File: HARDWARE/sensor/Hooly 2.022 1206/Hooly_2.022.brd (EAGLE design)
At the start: 33.4 x 25.4 mm, 34 parts, among them IC2 MCP1703CB, U3 MCP73831, U5 ATMEGA328P-AU

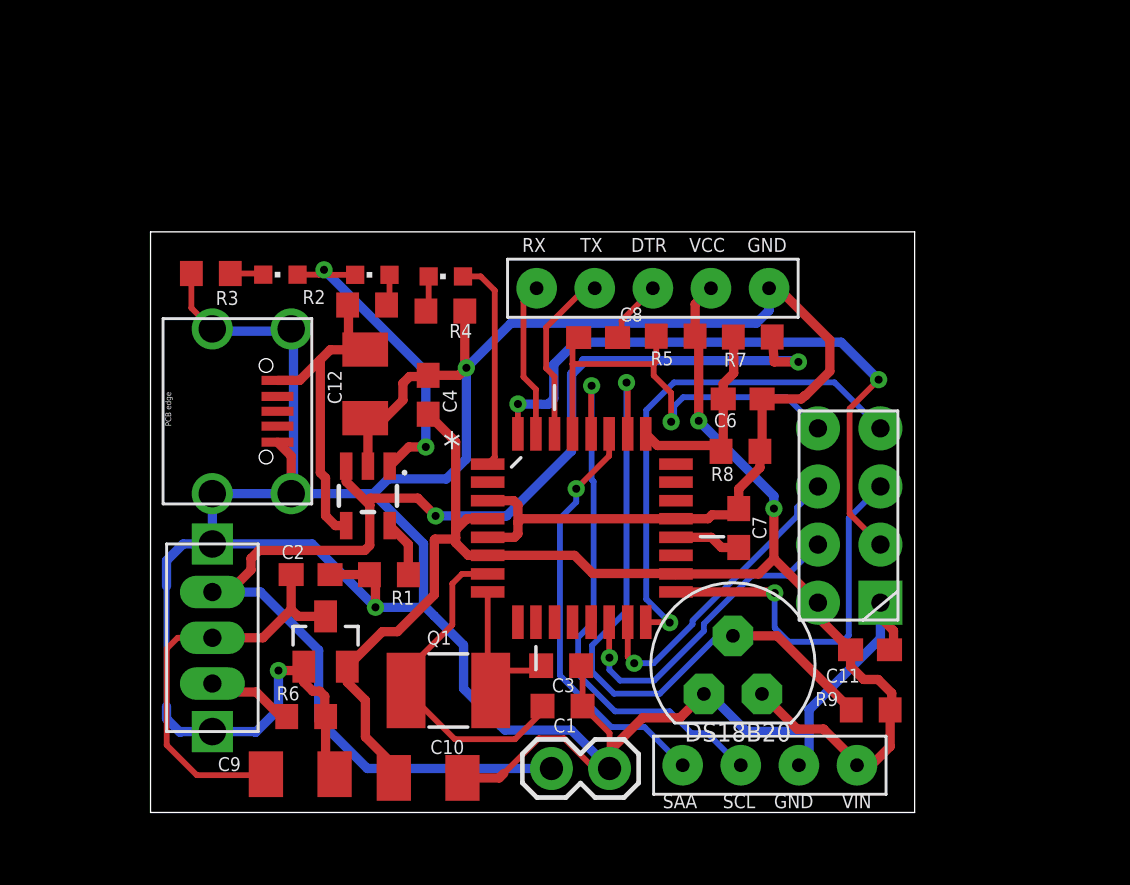
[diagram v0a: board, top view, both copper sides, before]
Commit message: Hardware update
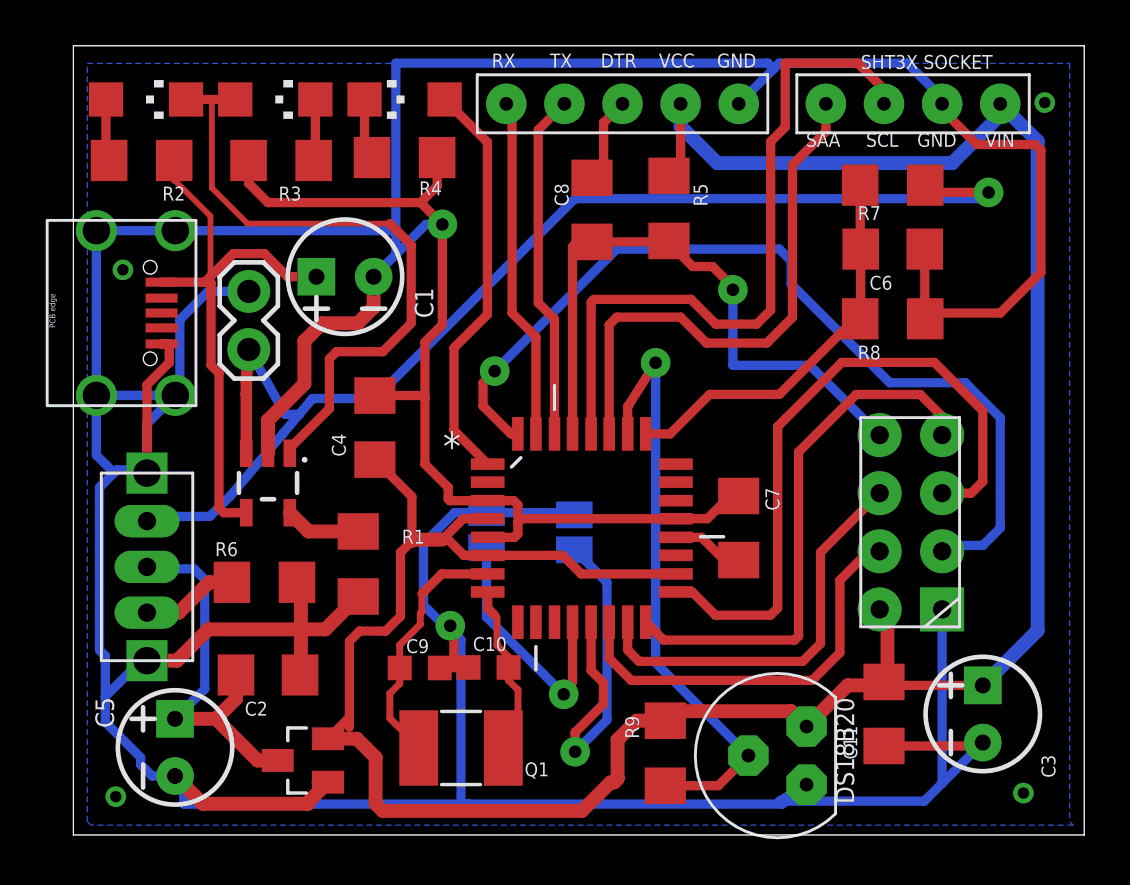
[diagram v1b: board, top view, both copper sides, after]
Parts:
- removed C12: (no value), resistor:C1206K
- added C5: 10uF, SparkFun-Capacitors:CPOL-RADIAL-2.5MM-5MM
- added SJ1, SJ2: (no value), jumper:SJ
- C1: value (none) -> 4.7uF; device rcl:C0603K -> SparkFun-Capacitors:CPOL-RADIAL-2.5MM-5MM
- C10, C9: value 1uF -> 22pF; device resistor:C1206K -> rcl:C0603K
- C11, C2, C4, C6, C7, C8: device resistor:C0603 -> resistor:C1206
- C3: value (none) -> 10uF; device rcl:C0603K -> SparkFun-Capacitors:CPOL-RADIAL-2.5MM-5MM
- LED1, LED2, LED4: device led:CHIPLED_0603 -> led:CHIPLED_1206
- Q1: value (none) -> 8MHz Crystal
- R1, R2, R3, R4, R5, R6, R7, R8, R9: device rcl:R0603 -> rcl:R1206
- moved U$1 29.6 mm to (34.8, 30.0)
- moved J2 26.1 mm to (8.30, 21.8), turned to 270 degrees
- moved C1 21.0 mm to (12.5, 22.4), turned to 180 degrees
- moved C3 18.6 mm to (40.4, 3.30), turned to 90 degrees
- moved LED1 12.5 mm to (3.81, 30.2), turned to 270 degrees
- moved R2 11.7 mm to (3.62, 27.5), turned to 180 degrees
- moved C6 9.27 mm to (36.4, 23.6)
- moved R9 9.18 mm to (26.5, 1.59), turned to 90 degrees
- moved R7 9.03 mm to (36.4, 26.4)
- moved R8 8.82 mm to (36.4, 20.6)
- moved U$6 8.17 mm to (20.8, 30.0)
- moved LED4 7.94 mm to (15.1, 30.2)
- moved LED2 7.66 mm to (9.46, 30.2), turned to 270 degrees
- moved C9 6.99 mm to (15.8, 5.31)
- moved R4 6.94 mm to (15.1, 27.6)
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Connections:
- net GND: now also C10.1, C3.2, C5.2, SJ1.1, SJ2.2; no longer C10.2, C12.2, C3.1
- net N$2: now also C5.1; no longer C9.1
- net SW1: now also SJ1.2
- net SW2: now also SJ2.1
- net VCC: now also C3.1; no longer C10.1
- net VUSB: now also C1.1; no longer C12.1
- net XTAL1: now also C9.1; no longer C1.1
- net XTAL2: now also C10.2; no longer C3.2
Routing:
- net GND: track 180.9 -> 277.6 mm, vias 3 -> 2
- net VCC: track 70.8 -> 117.3 mm, vias 2 -> 0
- net SW2: track 0.00 -> 16.4 mm, vias 0 -> 1
- net N$8: track 14.5 -> 28.2 mm, vias 2 -> 0
- net SCK: track 16.5 -> 29.0 mm, vias 1 -> 0
- net SW1: track 0.00 -> 11.1 mm, vias 0 -> 1
- net CE: track 28.9 -> 39.6 mm, vias 2 -> 1
- net VUSB: track 14.4 -> 25.0 mm
- net N$3: track 9.52 -> 17.9 mm
- net CKBAT: track 9.06 -> 17.3 mm
- net TX: track 6.87 -> 14.6 mm
- net RESET: track 19.7 -> 27.4 mm
- net RX: track 7.75 -> 15.3 mm
- net SCL: track 23.8 -> 30.8 mm, vias 1 -> 0
- net SDA: track 18.5 -> 23.8 mm, vias 1 -> 0
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- added copper zone on layer 16, net GND
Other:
- board size 33.4 x 25.4 mm -> 44.2 x 34.5 mm
- board text added: "GND"
- board text added: "SHT3X SOCKET"
